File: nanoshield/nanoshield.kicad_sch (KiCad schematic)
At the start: 8 parts, among them J1 Conn_01x20_Socket, J2 Joy, J3 Conn_01x20_Socket, J4 M0S, J5 MIDI OUT

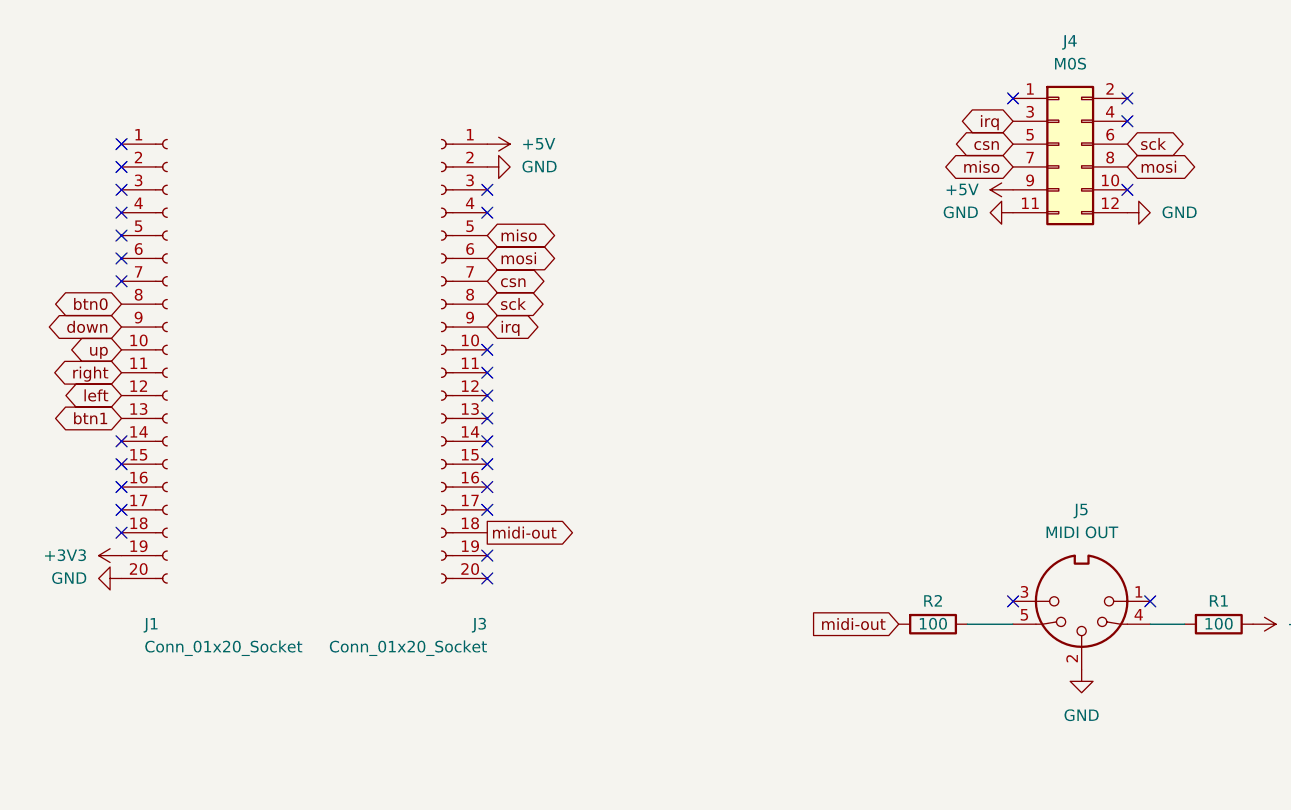
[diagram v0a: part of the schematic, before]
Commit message: added jlcpcb bom
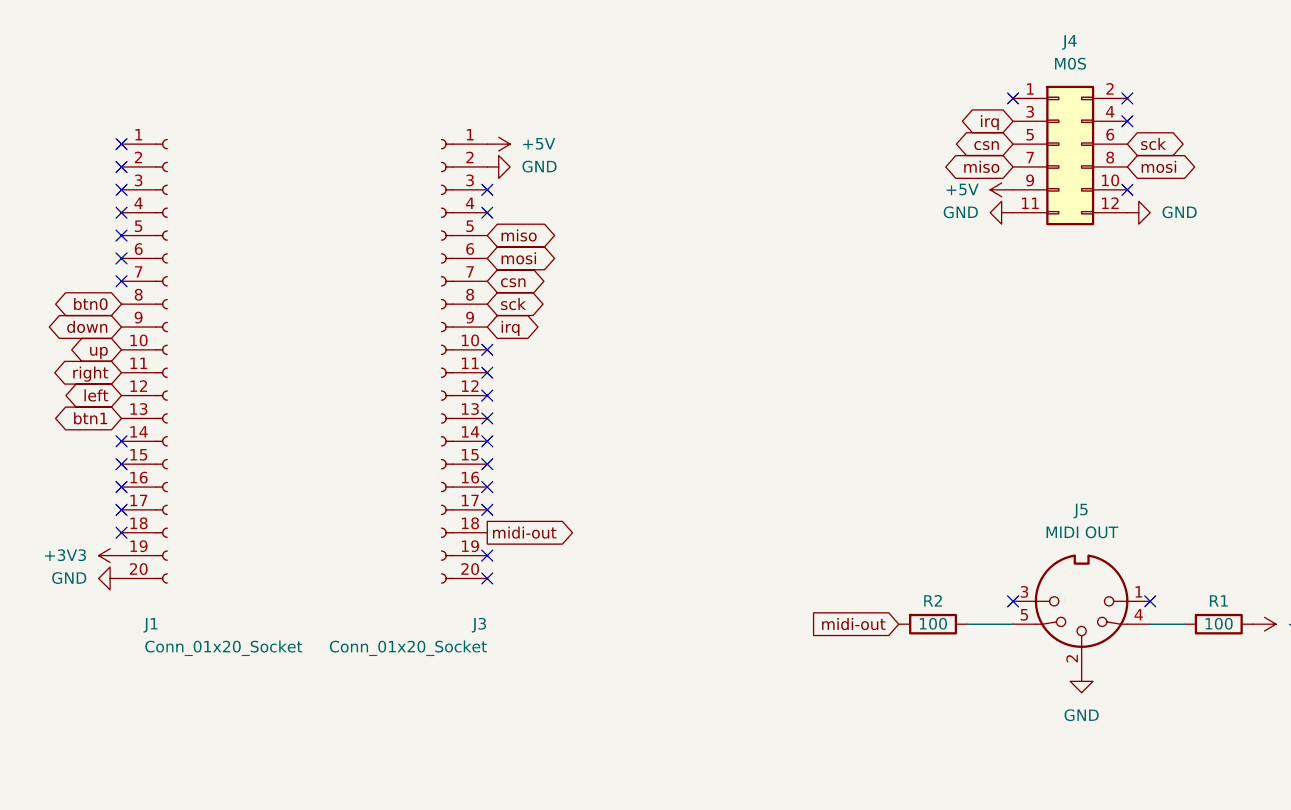
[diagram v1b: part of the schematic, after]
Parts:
- C1: LCSC Part # (none) -> C3009699
- J1, J3: LCSC Part # (none) -> C5224030
- J4: LCSC Part # (none) -> C5333437
- J5: LCSC Part # (none) -> C2939346
- R1, R2: LCSC Part # (none) -> C1364269
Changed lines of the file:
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@@
 (kicad_sch
-	(version 20231120)
+	(version 20250114)
 	(generator "eeschema")
-	(generator_version "8.0")
+	(generator_version "9.0")
 	(paper "A4")
 	(title_block
@@
 		(company "csynt")
 	)
+	(text "Shield for Tang Nano 20K/M0S dock (MiSTeryNano project)\n© 2024 C_Syntichakis <csynt8bit@gmail.com>"
+		(exclude_from_sim no)
+		(at 179.07 173.99 0)
+		(effects
+			(font
+				(face "KiCad Font")
+				(size 2 2)
+			)
+			(justify left bottom)
+			(href "https://github.com/uxware/nanoshield")
+		)
+	)
 	(no_connect
 		(at 121.92 78.74)
@@
 			(width 0)
 			(type default)
-		)
-	)
-	(text "Shield for Tang Nano 20K/M0S dock (MiSTeryNano project)\n© 2024 C_Syntichakis <csynt8bit@gmail.com>"
-		(exclude_from_sim no)
-		(at 179.07 173.99 0)
-		(effects
-			(font
-				(face "KiCad Font")
-				(size 2 2)
-			)
-			(justify left bottom)
-			(href "https://github.com/uxware/nanoshield")
 		)
 	)
@@
 			)
 		)
+		(property "LCSC Part #" "C5224030"
+			(at 86.36 55.88 0)
+			(effects
+				(font
+					(size 1.27 1.27)
+				)
+				(hide yes)
+			)
+		)
 		(pin "5"
 		)
@@
 			)
 		)
+		(property "LCSC Part #" "C1364269"
+			(at 203.2 86.36 90)
+			(effects
+				(font
+					(size 1.27 1.27)
+				)
+				(hide yes)
+			)
+		)
 		(pin "2"
 		)
@@
 		)
 		(property "Description" ""
+			(at 187.96 83.82 0)
+			(effects
+				(font
+					(size 1.27 1.27)
+				)
+				(hide yes)
+			)
+		)
+		(property "LCSC Part #" "C2939346"
 			(at 187.96 83.82 0)
 			(effects
@@
 			)
 		)
-		(property "Datasheet" " ~"
+		(property "Datasheet" "~"
 			(at 40.64 38.1 0)
 			(effects
@@
 		)
 		(property "Description" ""
+			(at 185.42 33.02 0)
+			(effects
+				(font
+					(size 1.27 1.27)
+				)
+				(hide yes)
+			)
+		)
+		(property "LCSC Part #" "C5333437"
 			(at 185.42 33.02 0)
 			(effects
@@
 			)
 		)
+		(property "LCSC Part #" "C1364269"
+			(at 171.45 86.36 90)
+			(effects
+				(font
+					(size 1.27 1.27)
+				)
+				(hide yes)
+			)
+		)
 		(pin "2"
 		)
@@
 		)
 		(property "Description" ""
+			(at 227.33 83.82 0)
+			(effects
+				(font
+					(size 1.27 1.27)
+				)
+				(hide yes)
+			)
+		)
+		(property "LCSC Part #" "C3009699"
 			(at 227.33 83.82 0)
 			(effects
@@
 			)
 		)
+		(property "LCSC Part #" "C5224030"
+			(at 116.84 55.88 0)
+			(effects
+				(font
+					(size 1.27 1.27)
+				)
+				(hide yes)
+			)
+		)
 		(pin "5"
 		)
@@
 		)
 	)
+	(embedded_fonts no)
 )
